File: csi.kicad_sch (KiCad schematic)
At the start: 1 part, among them J3 Conn_01x20

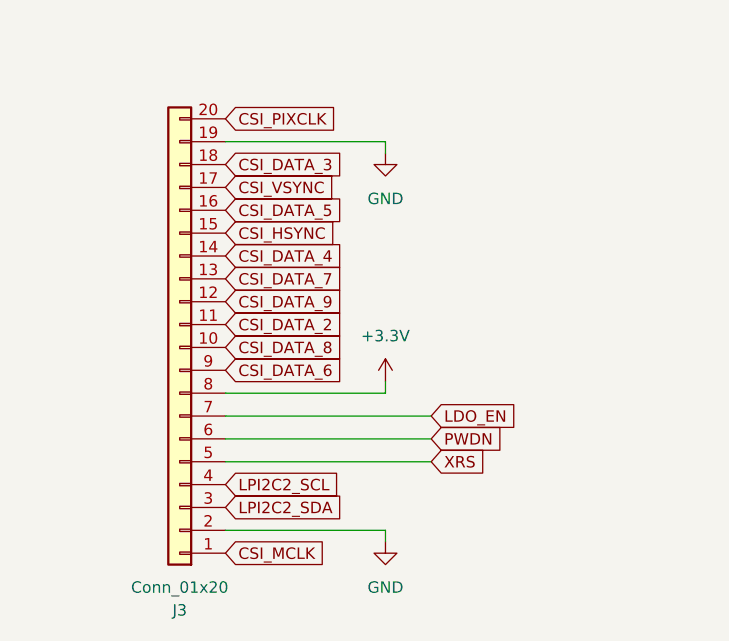
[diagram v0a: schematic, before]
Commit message: v0.2
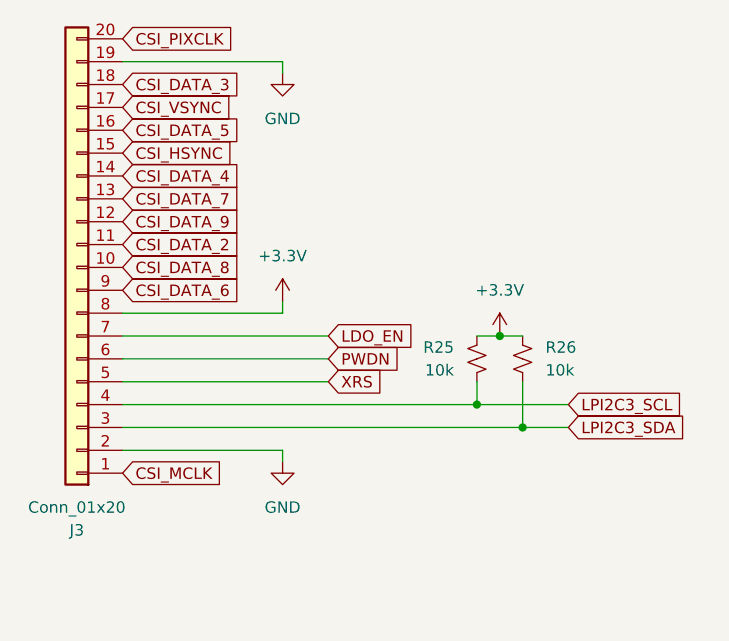
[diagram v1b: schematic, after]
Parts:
- added R25, R26: 10k, symbol Device:R_Small_US
- J3: footprint Connector_FFC-FPC:Molex_200528-0200_1x20-1MP_P1.00mm_Horizontal -> (none)
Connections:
- net +3.3V: now also R25.1, R26.1
- net LPI2C2_SCL renamed LPI2C3_SCL
- net LPI2C3_SCL: now also R25.2
- net LPI2C2_SDA renamed LPI2C3_SDA
- net LPI2C3_SDA: now also R26.2
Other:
- title: RT1050 DevBoard for Project Horizon -> Payload Board for Pleiades Atlas
- moved on the sheet: J3

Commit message: started layout
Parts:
- J3: footprint (none) -> Connector_FFC-FPC:TE_2-1734839-0_1x20-1MP_P0.5mm_Horizontal
- R25, R26: footprint (none) -> Resistor_SMD:R_0402_1005Metric
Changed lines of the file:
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@@
 			)
 		)
-		(property "Footprint" ""
+		(property "Footprint" "Connector_FFC-FPC:TE_2-1734839-0_1x20-1MP_P0.5mm_Horizontal"
 			(at 20.32 45.72 0)
 			(effects
@@
 			)
 		)
-		(property "Footprint" ""
+		(property "Footprint" "Resistor_SMD:R_0402_1005Metric"
 			(at 64.77 55.88 0)
 			(effects
@@
 			)
 		)
-		(property "Footprint" ""
+		(property "Footprint" "Resistor_SMD:R_0402_1005Metric"
 			(at 69.85 55.88 0)
 			(effects

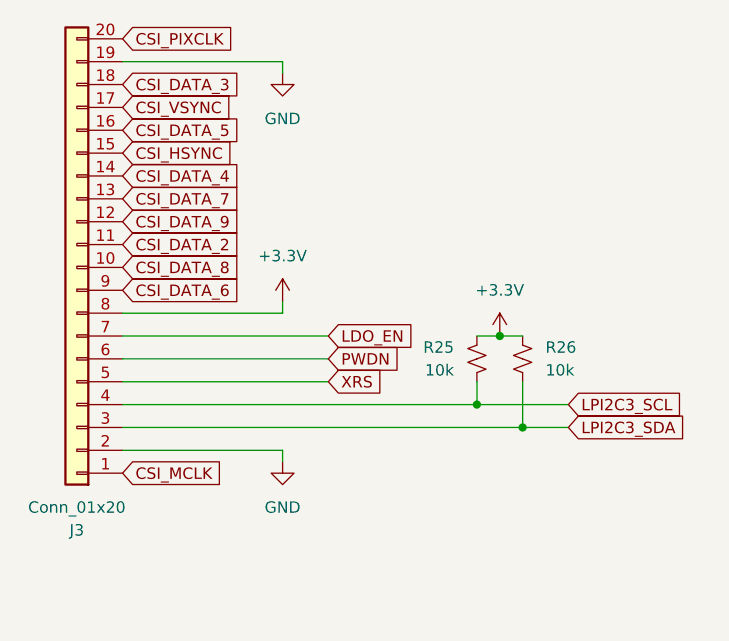
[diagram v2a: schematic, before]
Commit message: finished layout of v0.2!
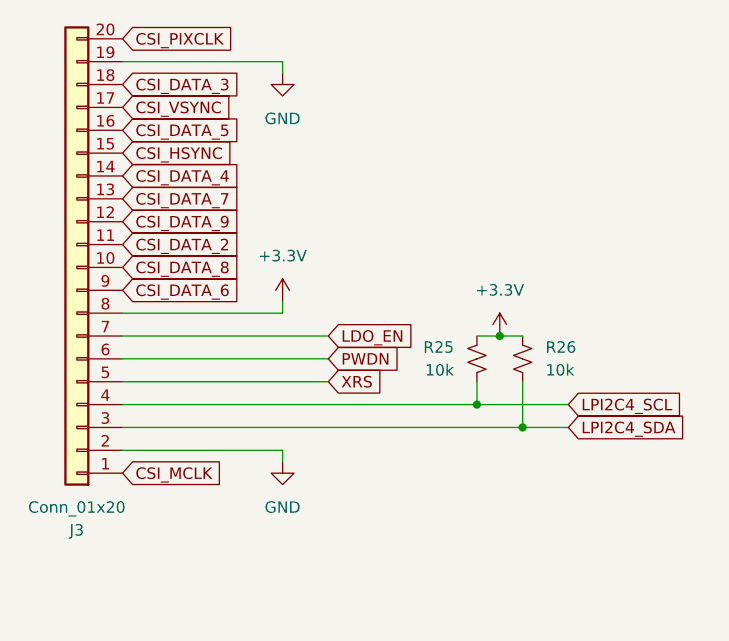
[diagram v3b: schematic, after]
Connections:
- net LPI2C3_SCL renamed LPI2C4_SCL
- net LPI2C3_SDA renamed LPI2C4_SDA
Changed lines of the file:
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@@
+		)
+	)
+	(global_label "LPI2C4_SDA"
+		(shape input)
+		(at 74.93 63.5 0)
+		(fields_autoplaced yes)
+		(effects
+			(font
+				(size 1.27 1.27)
+			)
+			(justify left)
+		)
+		(property "Intersheetrefs" "${INTERSHEET_REFS}"
+			(at 89.0428 63.5 0)
+			(effects
+				(font
+					(size 1.27 1.27)
+				)
+				(justify left)
+				(hide yes)
+			)
 		)
 	)
@@
 		)
 	)
+	(global_label "LPI2C4_SCL"
+		(shape input)
+		(at 74.93 60.96 0)
+		(fields_autoplaced yes)
+		(effects
+			(font
+				(size 1.27 1.27)
+			)
+			(justify left)
+		)
+		(property "Intersheetrefs" "${INTERSHEET_REFS}"
+			(at 88.9823 60.96 0)
+			(effects
+				(font
+					(size 1.27 1.27)
+				)
+				(justify left)
+				(hide yes)
+			)
+		)
+	)
 	(global_label "CSI_DATA_3"
 		(shape input)
@@
 		)
 	)
-	(global_label "LPI2C3_SDA"
-		(shape input)
-		(at 74.93 63.5 0)
-		(fields_autoplaced yes)
-		(effects
-			(font
-				(size 1.27 1.27)
-			)
-			(justify left)
-		)
-		(property "Intersheetrefs" "${INTERSHEET_REFS}"
-			(at 89.0428 63.5 0)
-			(effects
-				(font
-					(size 1.27 1.27)
-				)
-				(justify left)
-				(hide yes)
-			)
-		)
-	)
 	(global_label "CSI_DATA_8"
 		(shape input)
@@
 			(effects
 				(font
-					(size 1.27 1.27)
-				)
-				(justify left)
-				(hide yes)
-			)
-		)
-	)
-	(global_label "LPI2C3_SCL"
-		(shape input)
-		(at 74.93 60.96 0)
-		(fields_autoplaced yes)
-		(effects
-			(font
-				(size 1.27 1.27)
-			)
-			(justify left)
-		)
-		(property "Intersheetrefs" "${INTERSHEET_REFS}"
-			(at 88.9823 60.96 0)
-			(effects
-				(font
